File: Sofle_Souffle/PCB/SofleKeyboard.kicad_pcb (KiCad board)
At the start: 2 copper layers, 143.3 x 111.7 mm, 94 parts, among them J2 4PIN, J3 OLED, P3 i2c_pin, P4 i2c_pin, P5 i2c_pin, P6 i2c_pin, P7 i2c_pin, SW1 SW_PUSH-MX_W_LED, SW10 SW_PUSH-MX_W_LED, SW11 SW_PUSH-MX_W_LED, SW12 SW_PUSH-MX_W_LED, SW13 SW_PUSH-MX_W_LED, SW14 SW_PUSH-MX_W_LED, SW15 SW_PUSH-MX_W_LED, SW16 SW_PUSH-MX_W_LED, SW17 SW_PUSH-MX_W_LED, SW18 SW_PUSH-MX_W_LED, SW19 SW_PUSH-MX_W_LED, SW2 SW_PUSH-MX_W_LED, SW20 SW_PUSH-MX_W_LED, SW21 SW_PUSH-MX_W_LED, SW22 SW_PUSH-MX_W_LED, SW23 SW_PUSH-MX_W_LED, SW24 SW_PUSH-MX_W_LED, SW25 Rotary_Encoder_Switch, SW25A1 SW_PUSH-MX_W_LED, SW26 SW_PUSH-MX_W_LED, SW27 SW_PUSH-MX_W_LED, SW28 SW_PUSH-MX_W_LED, SW29 SW_PUSH-MX_W_LED, SW3 SW_PUSH-MX_W_LED, SW30 SW_PUSH-MX_W_LED, SW4 SW_PUSH-MX_W_LED, SW5 SW_PUSH-MX_W_LED, SW6 SW_PUSH-MX_W_LED, SW7 SW_PUSH-MX_W_LED, SW8 SW_PUSH-MX_W_LED, SW9 SW_PUSH-MX_W_LED, U1 ProMicro

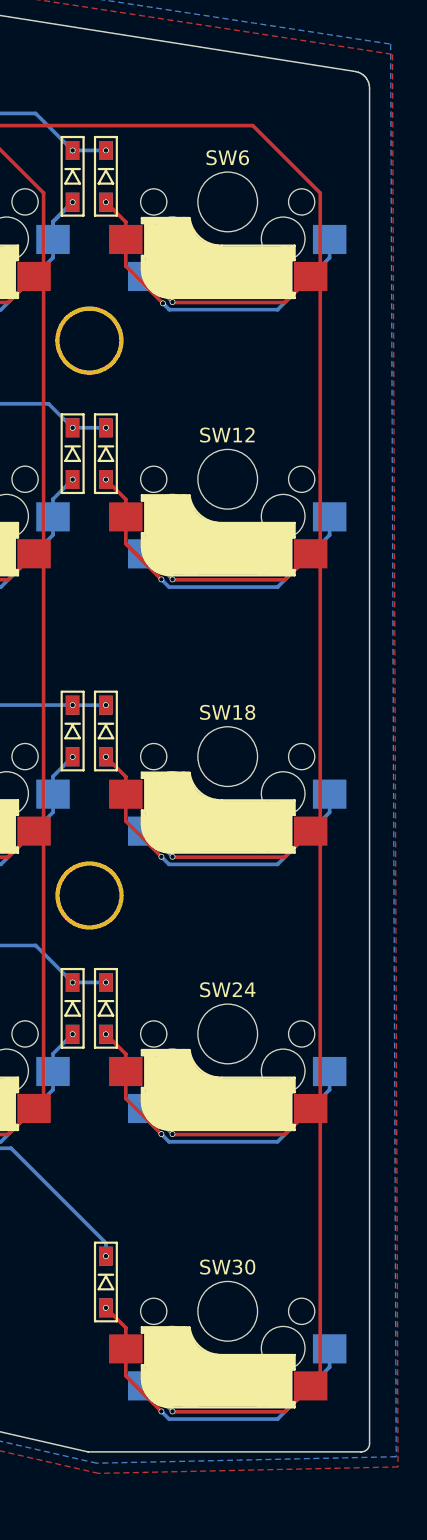
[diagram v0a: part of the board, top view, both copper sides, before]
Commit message: Checkpoint commit.
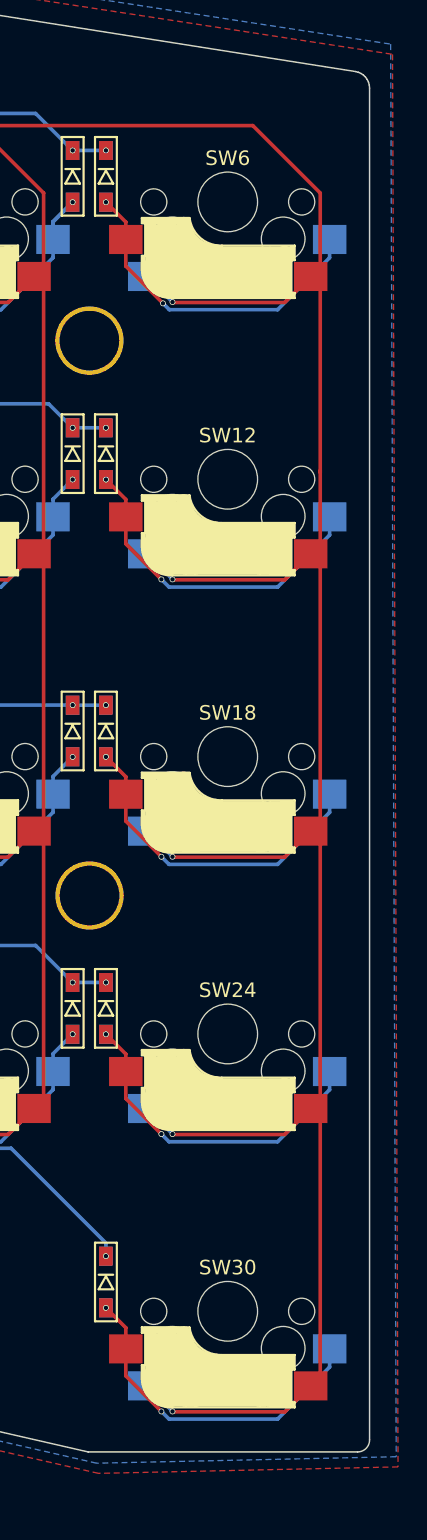
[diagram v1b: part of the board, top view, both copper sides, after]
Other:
- outline, holes or cut-outs redrawn
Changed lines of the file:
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@@
   (setup
     (pad_to_mask_clearance 0)
-    (grid_origin 90.424 80.01)
+    (grid_origin 93.218 106.934)
     (pcbplotparams
       (layerselection 0x00010fc_ffffffff)
@@
     (fp_line (start 5.9 -1.1) (end 2.62 -1.1) (layer "F.SilkS") (width 0.15))
     (fp_line (start 5.67 -3.7) (end 5.67 -1.46) (layer "F.SilkS") (width 0.15))
-    (fp_arc (start 0.8 -3.4) (mid 2.26871 -2.886118) (end 3.016318 -1.521471) (layer "F.SilkS") (width 1))
+    (fp_arc (start 0.8 -3.4) (mid 2.268709 -2.886118) (end 3.016318 -1.521471) (layer "F.SilkS") (width 1))
     (fp_arc (start 0.4 -3) (mid 1.868709 -2.486118) (end 2.616318 -1.121471) (layer "F.SilkS") (width 0.15))
     (fp_arc (start 3.8 -6.600001) (mid 5.243504 -6.084925) (end 5.900001 -4.7) (layer "F.SilkS") (width 0.15))
@@
     )
   )
-  (gr_line (start 218.769181 46.770902) (end 218.768802 139.879974) (layer "Cmts.User") (width 0.1))
-  (gr_arc (start 218.768802 139.879974) (mid 218.600311 140.284023) (end 218.194741 140.448819) (layer "Cmts.User") (width 0.1))
-  (gr_line (start 218.194741 140.448819) (end 199.4343 140.44882) (layer "Cmts.User") (width 0.1))
+  (gr_line (start 218.769181 46.770902) (end 218.768802 139.625974) (layer "Cmts.User") (width 0.1))
+  (gr_line (start 217.940741 140.448819) (end 199.4343 140.44882) (layer "Cmts.User") (width 0.1))
   (gr_line (start 218.352621 45.8846) (end 218.494321 46.024582) (layer "Cmts.User") (width 0.1))
   (gr_line (start 142.326 37.189) (end 164.276 37.189) (layer "Cmts.User") (width 0.1))
@@
   (gr_line (start 131.480128 136.189) (end 180.826 136.189) (layer "Cmts.User") (width 0.1))
   (gr_line (start 87.112 148.905) (end 87.54872 148.85416) (layer "Cmts.User") (width 0.1))
+  (gr_arc (start 218.768802 139.625974) (mid 218.526451 140.210164) (end 217.940741 140.448819) (layer "Cmts.User") (width 0.1))
   (gr_line (start 131.480128 136.189) (end 180.826 136.189) (layer "Edge.Cuts") (width 0.1))
   (gr_line (start 199.4343 140.44882) (end 180.826 136.189) (layer "Edge.Cuts") (width 0.1))
@@
   (gr_line (start 218.750381 46.563571) (end 218.769181 46.770902) (layer "Edge.Cuts") (width 0.1))
   (gr_line (start 85.876 148.389) (end 75.626 130.589) (layer "Edge.Cuts") (width 0.1))
-  (gr_line (start 218.194741 140.448819) (end 199.4343 140.44882) (layer "Edge.Cuts") (width 0.1))
-  (gr_arc (start 218.768802 139.879974) (mid 218.600311 140.284023) (end 218.194741 140.448819) (layer "Edge.Cuts") (width 0.1))
-  (gr_line (start 218.769181 46.770902) (end 218.768802 139.879974) (layer "Edge.Cuts") (width 0.1))
+  (gr_line (start 217.940741 140.448819) (end 199.4343 140.44882) (layer "Edge.Cuts") (width 0.1))
+  (gr_arc (start 218.768802 139.625974) (mid 218.5264 140.210113) (end 217.940741 140.448819) (layer "Edge.Cuts") (width 0.1))
+  (gr_line (start 218.769181 46.770902) (end 218.768802 139.625974) (layer "Edge.Cuts") (width 0.1))
   (gr_line (start 81.623257 40.434261) (end 81.690377 40.218014) (layer "Edge.Cuts") (width 0.1))
   (gr_line (start 164.276 37.189) (end 217.801441 45.634146) (layer "Edge.Cuts") (width 0.1))
